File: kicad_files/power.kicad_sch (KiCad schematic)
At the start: 23 parts, among them J8 Conn_01x02_Socket, Q1 FDMC510P-MS, SW3 SW_SPST, U11 LT1963AxST-3.3, U12 AP63205WU

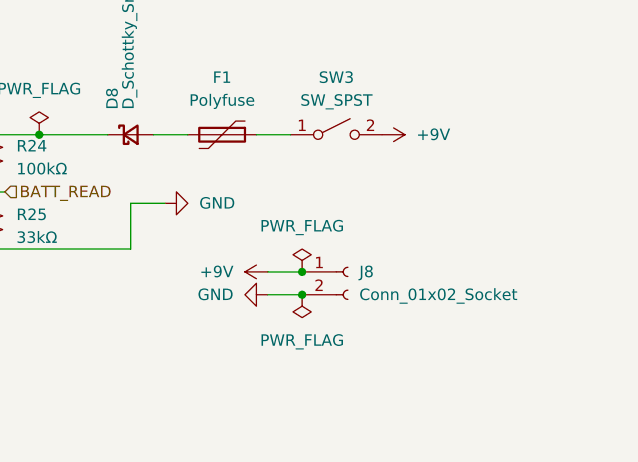
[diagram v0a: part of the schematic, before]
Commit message: Rearrange PCB
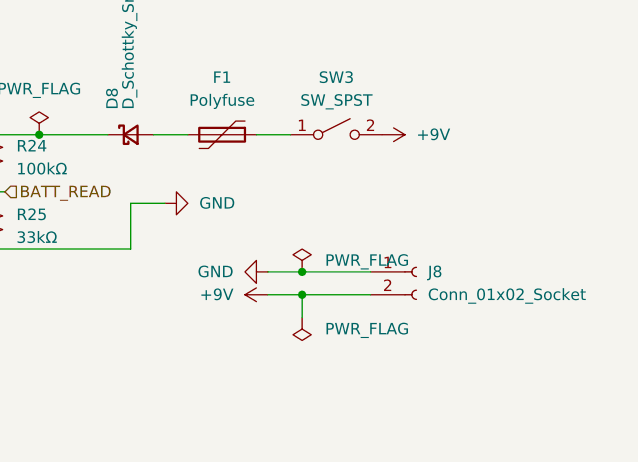
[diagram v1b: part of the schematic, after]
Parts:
- J8: footprint (none) -> Connector_AMASS:AMASS_XT30U-F_1x02_P5.0mm_Vertical
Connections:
- net +9V: now also J8.2 (Pin_2); no longer J8.1 (Pin_1)
- net GND: now also J8.1 (Pin_1); no longer J8.2 (Pin_2)
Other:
- moved on the sheet: J8
